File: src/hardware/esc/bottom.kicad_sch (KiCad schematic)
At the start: 64 parts, among them J10 Conn_01x01, J11 Conn_01x01, J12 Conn_01x01, J9 Conn_01x01, U10 STM32F051K8U6, U11 FD6288Q_C328453, U13 STM32F051K8U6, U14 FD6288Q_C328453, U6 INA2180A1

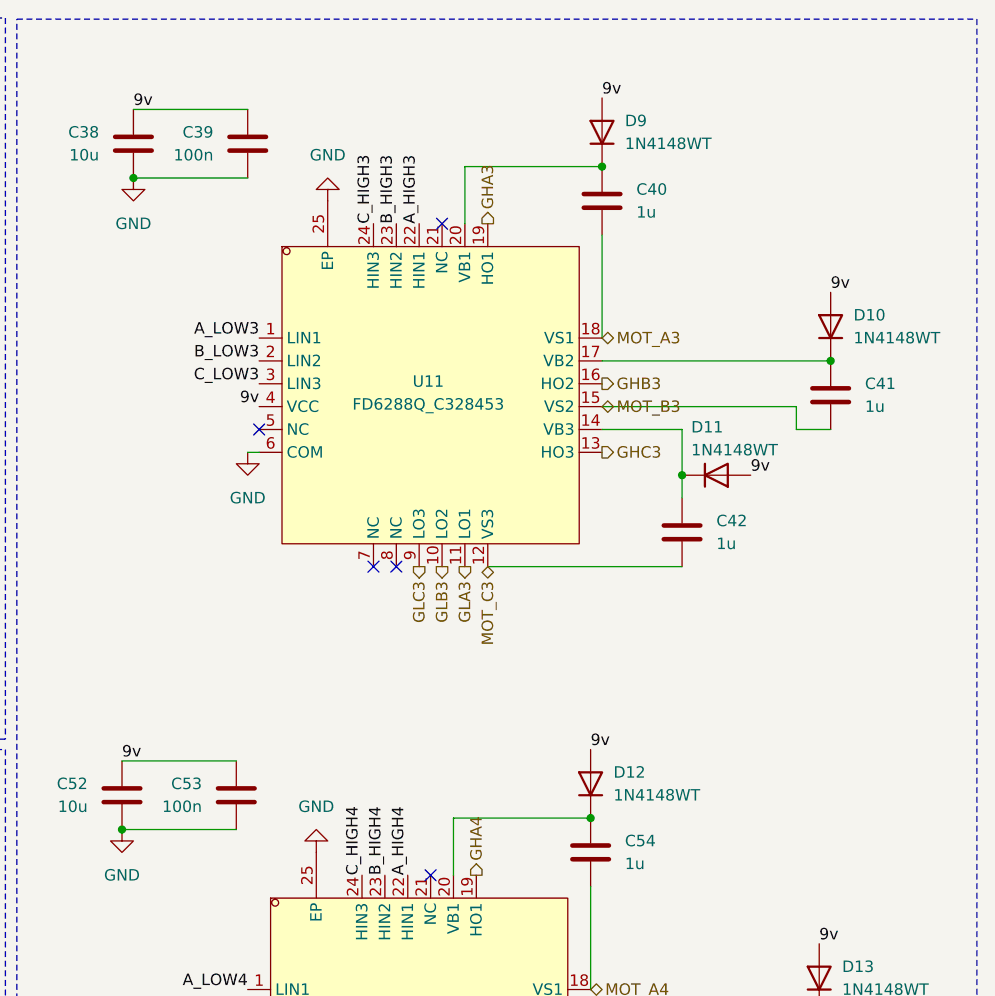
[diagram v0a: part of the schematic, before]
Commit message: a
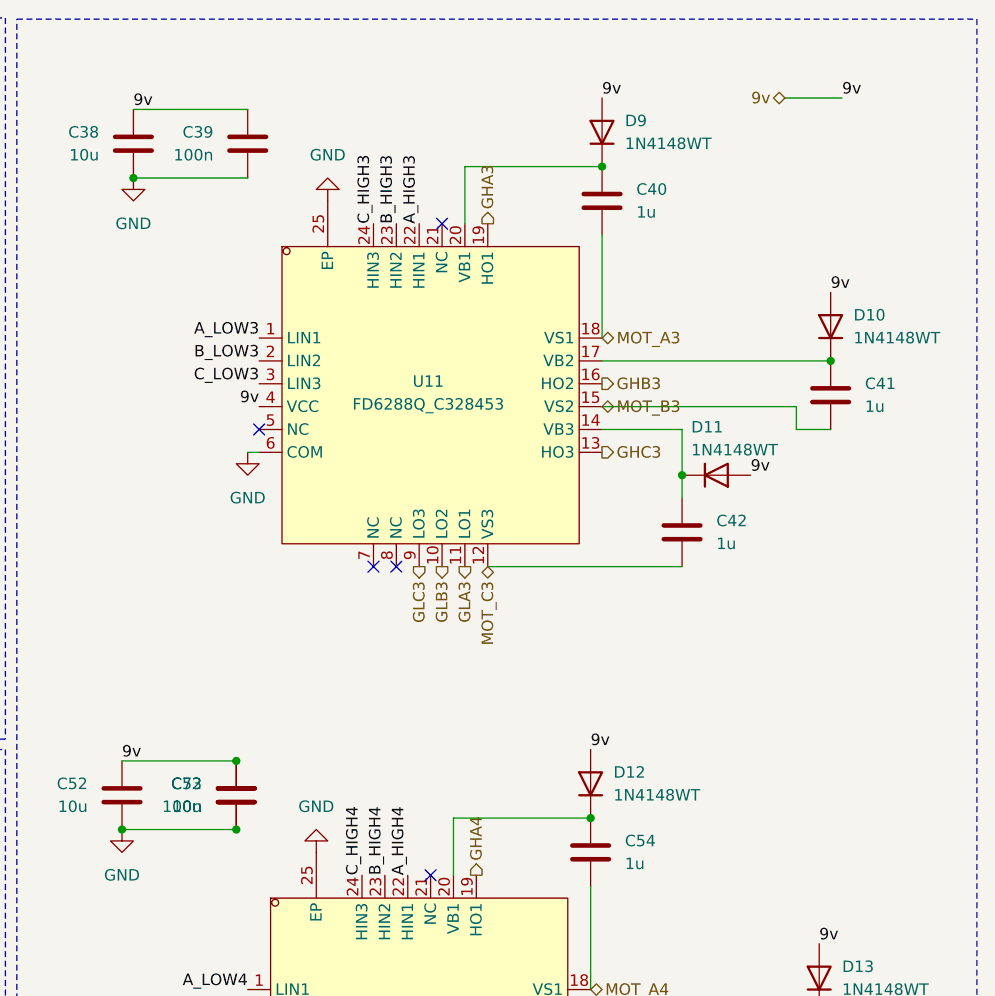
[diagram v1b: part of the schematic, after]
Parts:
- added C72: 10u, Capacitor_SMD:C_0603_1608Metric, symbol Device:C
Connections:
- net 9v: now also C72.1
- net GND: now also C72.2
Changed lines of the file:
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@@
 	)
 	(junction
+		(at 200.66 96.52)
+		(diameter 0)
+		(color 0 0 0 0)
+	)
+	(junction
 		(at 50.8 106.68)
 		(diameter 0)
@@
 	)
 	(junction
+		(at 200.66 104.14)
+		(diameter 0)
+		(color 0 0 0 0)
+	)
+	(junction
 		(at 27.94 78.74)
 		(diameter 0)
@@
 	(wire
 		(pts
+			(xy 267.97 22.86) (xy 261.62 22.86)
+		)
+		(stroke
+			(width 0)
+			(type default)
+		)
+	)
+	(wire
+		(pts
 			(xy 27.94 78.74) (xy 17.78 78.74)
 		)
@@
 		)
 	)
+	(label "9v"
+		(at 267.97 22.86 0)
+		(effects
+			(font
+				(size 1.27 1.27)
+			)
+			(justify left bottom)
+		)
+	)
 	(label "C_HIGH3"
 		(at 215.9 36.83 90)
@@
 		)
 	)
+	(hierarchical_label "9v"
+		(shape bidirectional)
+		(at 261.62 22.86 180)
+		(effects
+			(font
+				(size 1.27 1.27)
+			)
+			(justify right)
+		)
+	)
 	(hierarchical_label "GLA3"
 		(shape output)
@@
 					(unit 1)
 				)
+			)
+		)
+	)
+	(symbol
+		(lib_id "Device:C")
+		(at 200.66 100.33 0)
+		(mirror y)
+		(unit 1)
+		(body_style 1)
+		(exclude_from_sim no)
+		(in_bom yes)
+		(on_board yes)
+		(in_pos_files yes)
+		(dnp no)
+		(property "Reference" "C72"
+			(at 196.85 99.0599 0)
+			(show_name no)
+			(do_not_autoplace no)
+			(effects
+				(font
+					(size 1.27 1.27)
+				)
+				(justify left)
+			)
+		)
+		(property "Value" "10u"
+			(at 196.85 101.5999 0)
+			(show_name no)
+			(do_not_autoplace no)
+			(effects
+				(font
+					(size 1.27 1.27)
+				)
+				(justify left)
+			)
+		)
+		(property "Footprint" "Capacitor_SMD:C_0603_1608Metric"
+			(at 199.6948 104.14 0)
+			(hide yes)
+			(show_name no)
+			(do_not_autoplace no)
+			(effects
+				(font
+					(size 1.27 1.27)
+				)
+			)
+		)
+		(property "Datasheet" ""
+			(at 200.66 100.33 0)
+			(hide yes)
+			(show_name no)
+			(do_not_autoplace no)
+			(effects
+				(font
+					(size 1.27 1.27)
+				)
+			)
+		)
+		(property "Description" "Unpolarized capacitor"
+			(at 200.66 100.33 0)
+			(hide yes)
+			(show_name no)
+			(do_not_autoplace no)
+			(effects
+				(font
+					(size 1.27 1.27)
+				)
+			)
+		)
+		(property "LCSC" ""
+			(at 200.66 100.33 0)
+			(hide yes)
+			(show_name no)
+			(do_not_autoplace no)
+			(effects
+				(font
+					(size 1.27 1.27)
+				)
+			)
+		)
+		(pin "2"
+		)
+		(pin "1"
+		)
+		(instances
+			(project "esc"
+				(path "/7abcc5dd-3ad1-4c74-aa5d-e1502c746dfd/4ab5f7bf-96fa-4a0d-bad3-d50222998c4e"
+					(reference "C72")
+					(unit 1)
+				)

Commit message: a
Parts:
- C31, C45: LCSC C13585 -> C3039694
- C38, C52, C72: LCSC (none) -> C962136
- D10, D11, D12, D13, D14, D9: LCSC (none) -> C917006
- J10, J11, J12, J9: LCSC (none) -> x
- R44, R53, R54, R55, R63, R64, R73, R74, R75, R83: LCSC (none) -> C445596
- R45, R46, R47, R48, R49, R50, R65, R66, R67, R68, R69, R70, R71, R72: LCSC (none) -> C190095
- U6: LCSC (none) -> C2873353
